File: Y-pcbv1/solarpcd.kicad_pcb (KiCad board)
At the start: 6 copper layers, 64 x 58 mm, 56 parts, among them IC2 TSL2561, J1 XF2M-1015-1A, J2 U.FL-R-SMT-1, J3 BATTERY CONNECTOR, U1 SWLP.12.B, U2 Value, U3 SW_SPDT, U4 SW_SPDT

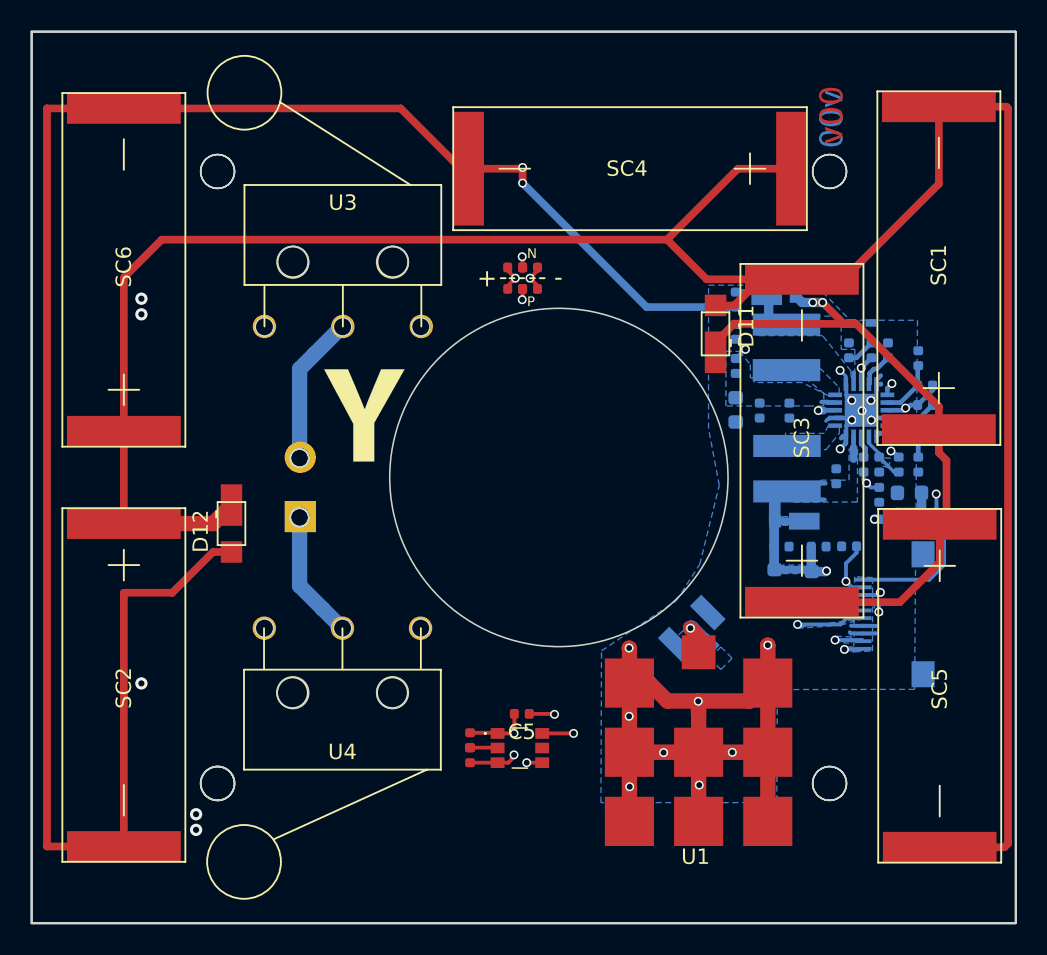
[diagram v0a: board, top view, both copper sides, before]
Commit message: Modified -Y Layout
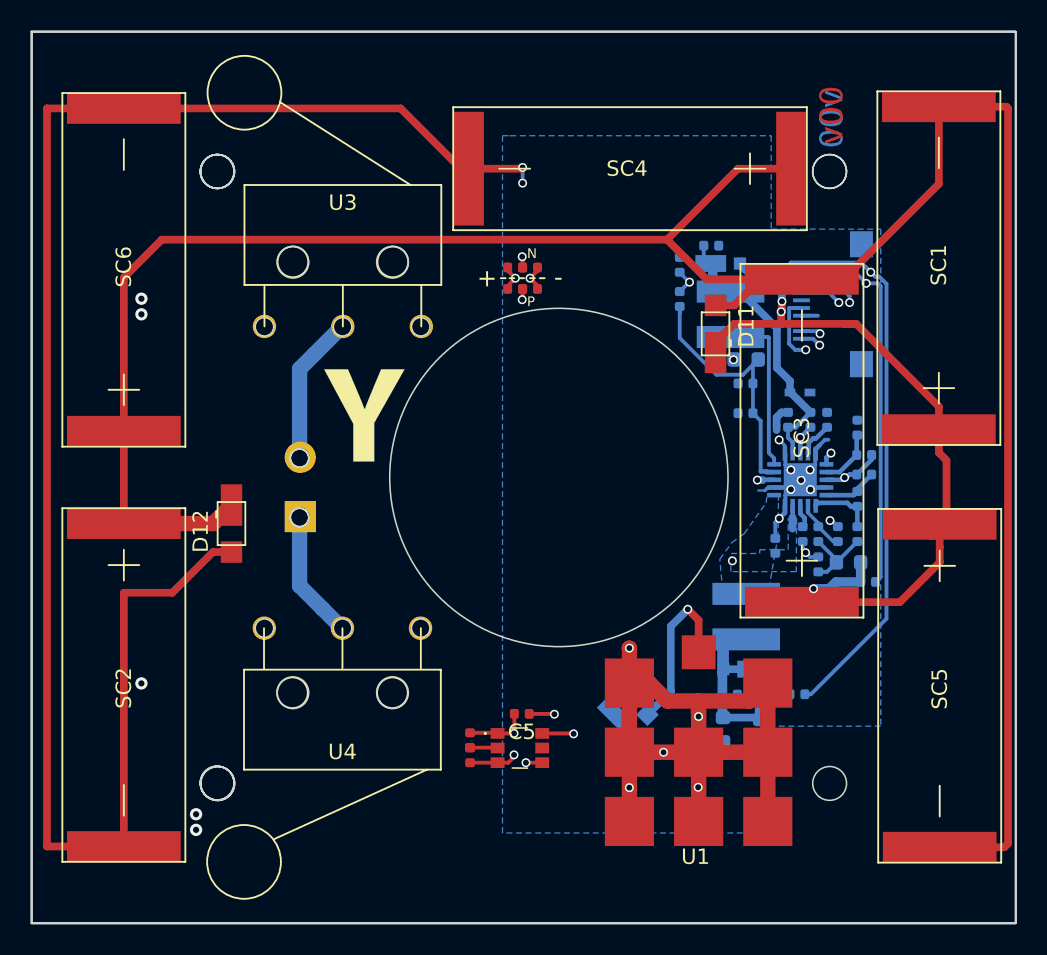
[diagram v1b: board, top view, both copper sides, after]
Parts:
- moved J1 20.6 mm to (163.1, 87.7)
- moved C13 10.2 mm to (160.4, 115.5)
- moved D2 10.2 mm to (159.2, 111.5)
- moved R15 10.2 mm to (162.8, 113.1)
- moved C12 10.2 mm to (158.0, 115.4)
- moved C14 10.2 mm to (160.8, 113.1)
- moved C10 10.2 mm to (158.4, 113.1)
- moved L2 9.98 mm to (159.5, 108.0)
- moved C3 6.01 mm to (162.2, 95.3)
- moved C4 6.01 mm to (164.7, 95.3)
- moved D1 6.01 mm to (162.9, 93.5)
- moved J2 6.01 mm to (152.0, 113.4)
- moved R11 6.01 mm to (163.7, 95.3)
- moved R14 6.01 mm to (167.4, 105.8)
- moved R3 6.01 mm to (166.7, 95.8)
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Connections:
- C10 pad 1: +3V3 -> GND
- C12 pad 1: +3V3 -> GND
- C13 pad 1: +3V3 -> GND
- C14 pad 1: +3V3 -> GND
- D2 pad 1: +3V3 -> GND
- D2 pad 2: +3V3 -> GND
- L2 pad 2: +3V3 -> GND
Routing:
- net BATT_N: track 46.6 -> 100.8 mm
- net COIL_N: track 71.4 -> 23.4 mm
- net COIL_P: track 67.6 -> 22.6 mm
- net SCL1: track 29.5 -> 49.6 mm
- net SDA1: track 27.0 -> 45.6 mm
- net Net-(C11-Pad1): track 0.89 -> 17.1 mm
- net VSOLAR: track 6.82 -> 18.7 mm
- net Net-(L1-Pad2): track 0.00 -> 10.9 mm
- net Net-(R11-Pad1): track 12.0 -> 22.1 mm
- net GND: track 207.7 -> 199.1 mm, vias 19 -> 17
- net +3V3: track 53.7 -> 45.3 mm
- net Net-(J2-Pad3): track 3.40 -> 11.0 mm
- net Net-(D11-Pad1): track 44.6 -> 46.0 mm
- net BATT_P: track 68.6 -> 67.7 mm
- removed copper zone on B.Cu, net Net-(C11-Pad1)
- removed copper zone on B.Cu, net Net-(L1-Pad2)
- removed copper zone on B.Cu, net VSOLAR
